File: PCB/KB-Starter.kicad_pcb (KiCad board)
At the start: 2 copper layers, 97.1 x 101.4 mm, 67 parts, among them J1 USB_C_Receptacle_USB2.0, J2 SWD, SW1 SW_Push, U1 W25Q128JVS, U2 USBLC6-2SC6, U3 XC6206PxxxMR, U5 RP2040, Y1 12MHz

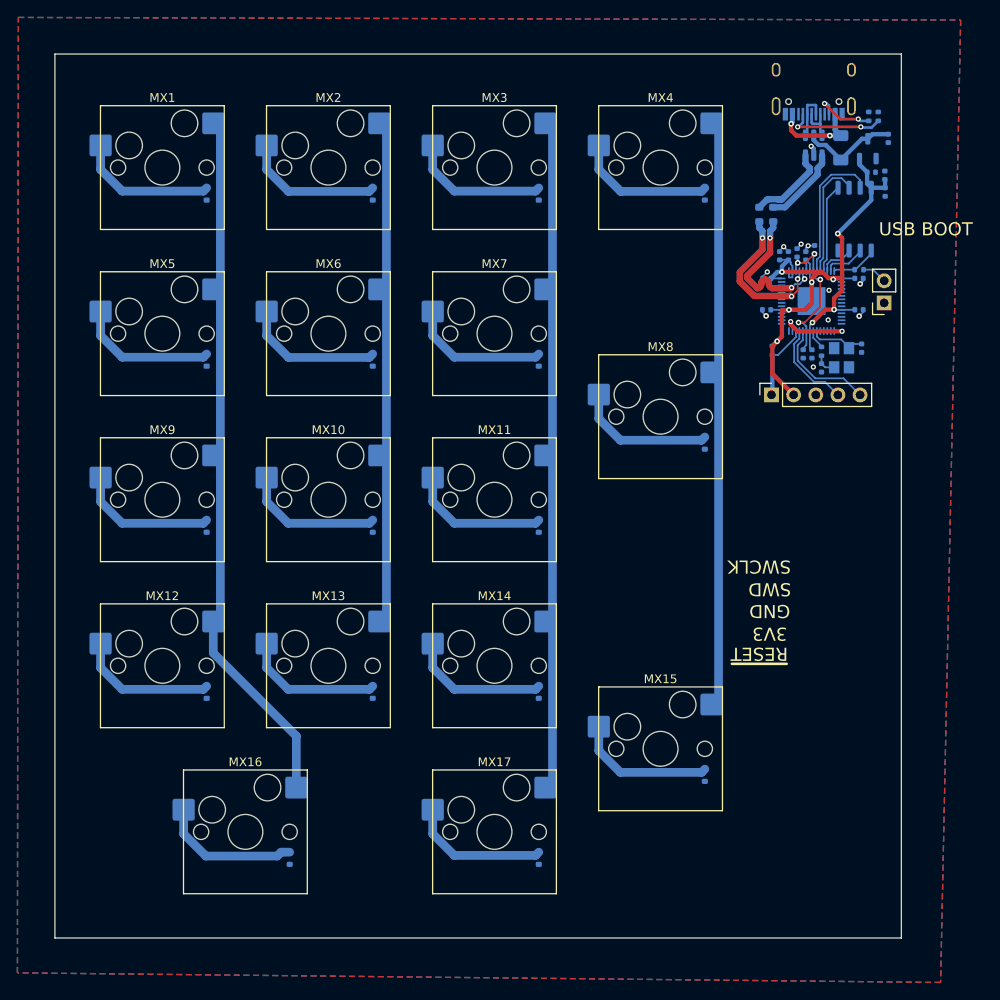
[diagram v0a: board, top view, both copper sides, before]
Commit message: fix+feat: matrix fix + touchup
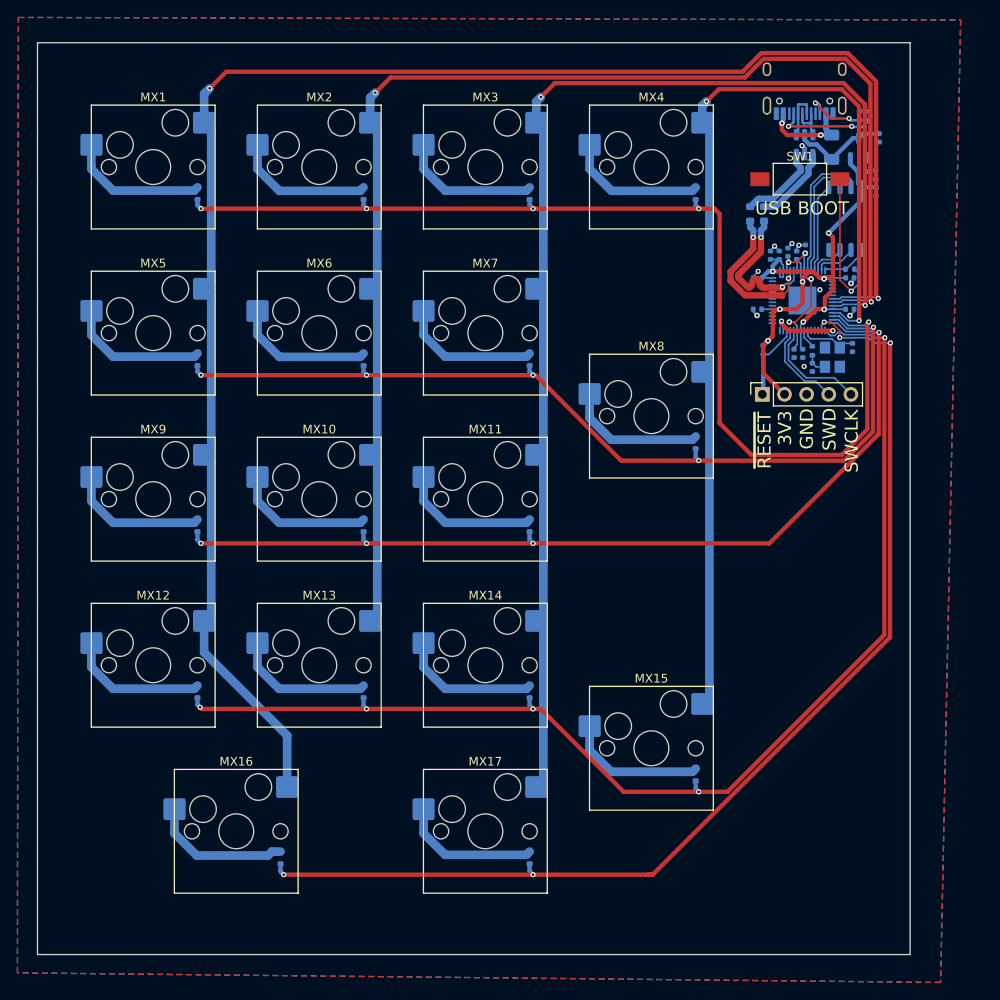
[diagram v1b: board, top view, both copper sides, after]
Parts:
- SW1: footprint Connector_PinSocket_2.54mm:PinSocket_1x02_P2.54mm_Vertical -> Button_Switch_SMD:SW_SPST_FSMSM
- moved SW1 17.2 mm to (107.7, 35.9), turned to 0 degrees
- moved C10 1.05 mm to (107.3, 44.6)
- moved C11 1.05 mm to (104.3, 44.6)
- moved C15 1.05 mm to (102.8, 50.8)
- moved C4 1.05 mm to (106.3, 44.2)
- moved C5 1.05 mm to (108.3, 43.9)
- moved C7 1.05 mm to (116.3, 35.3)
- moved C8 1.05 mm to (105.3, 44.6)
- moved J2 1.05 mm to (103.3, 60.5)
- moved R1 1.05 mm to (113.4, 46.2)
- moved R3 1.05 mm to (115.6, 28.6)
- moved D10 1.05 mm to (57.6, 75.6)
- moved D2 1.05 mm to (57.6, 37.5)
- moved D6 1.05 mm to (57.6, 56.5)
- moved MX2 1.05 mm to (52.5, 34.5)
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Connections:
- MX15 pad 2: Net-(MX15-Pad2) -> COL4
- MX4 pad 2: Net-(MX15-Pad2) -> COL4
- MX8 pad 2: Net-(MX15-Pad2) -> COL4
- U5 pad 11: COL3 -> COL4
- U5 pad 7: /GPIO5 -> COL1
- U5 pad 8: COL1 -> COL2
- U5 pad 9: COL2 -> COL3
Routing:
- net ROW4: track 0.00 -> 137.1 mm, vias 0 -> 5
- net ROW5: track 0.00 -> 128.2 mm, vias 0 -> 5
- net ROW1: track 0.00 -> 125.4 mm, vias 0 -> 5
- net COL4: track 0.00 -> 117.6 mm, vias 0 -> 2
- net COL1: track 82.2 -> 196.3 mm, vias 0 -> 2
- net ROW2: track 0.00 -> 105.0 mm, vias 0 -> 5
- net ROW3: track 0.00 -> 104.9 mm, vias 0 -> 4
- net COL2: track 59.2 -> 152.2 mm, vias 0 -> 2
- net COL3: track 78.9 -> 147.9 mm, vias 0 -> 2
- net Net-(MX15-Pad2): track 68.0 -> 0.00 mm
- net /~{USB_BOOT}: track 2.89 -> 16.5 mm, vias 0 -> 1
- net USBD_P: track 17.4 -> 17.2 mm, vias 3 -> 2
- net USBD_N: vias 3 -> 2
- net GND: vias 13 -> 12
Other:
- board size 97.1 x 101.4 mm -> 100.1 x 104.6 mm
